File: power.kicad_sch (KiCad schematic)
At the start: 32 parts, among them U2 XC6193A103ER-G, U3 TPS631000DRLR, U4 TPS62840DLCR, U5 BQ25185DLHR

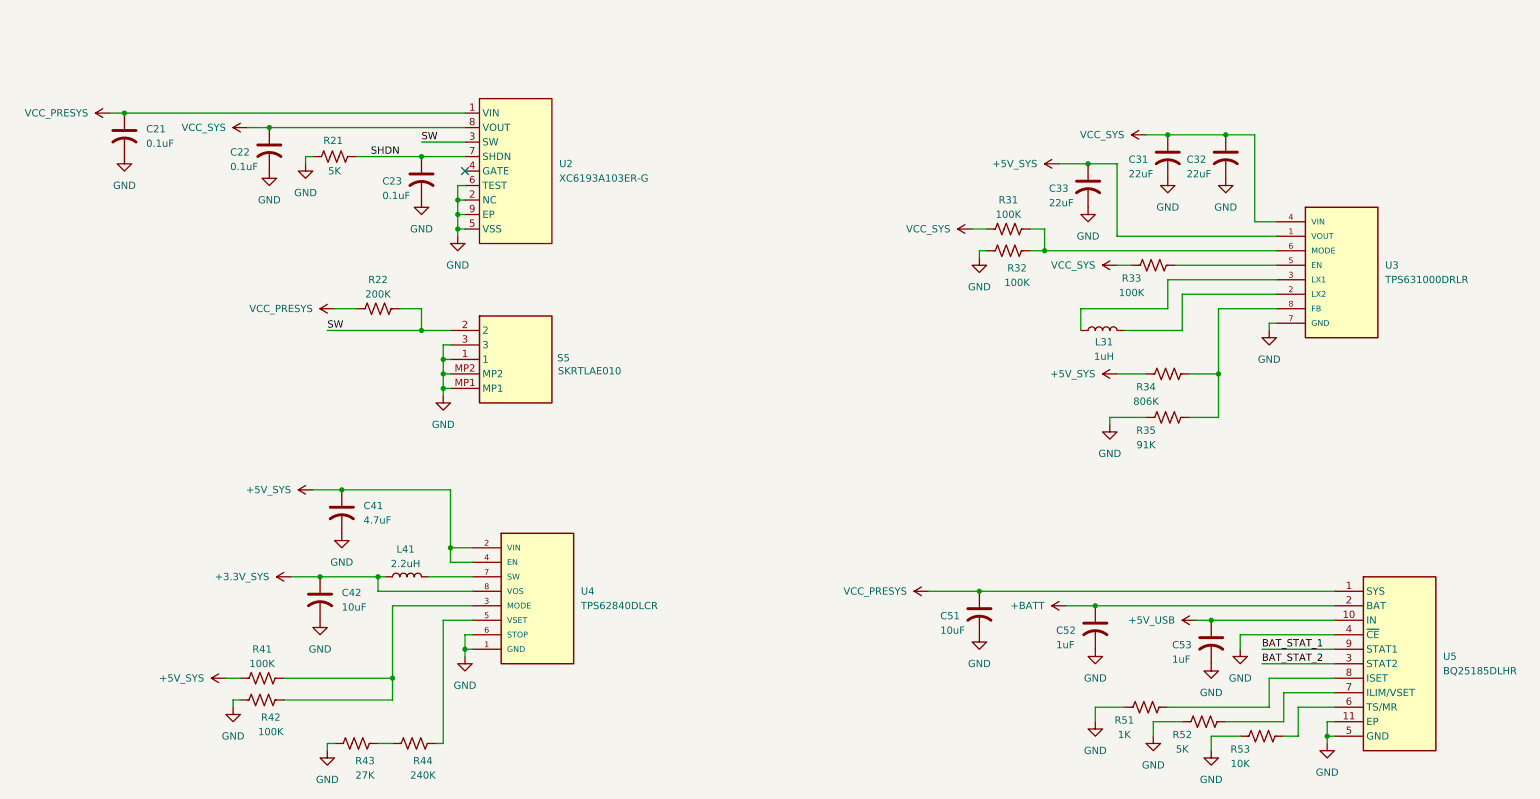
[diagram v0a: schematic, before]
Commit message: Update
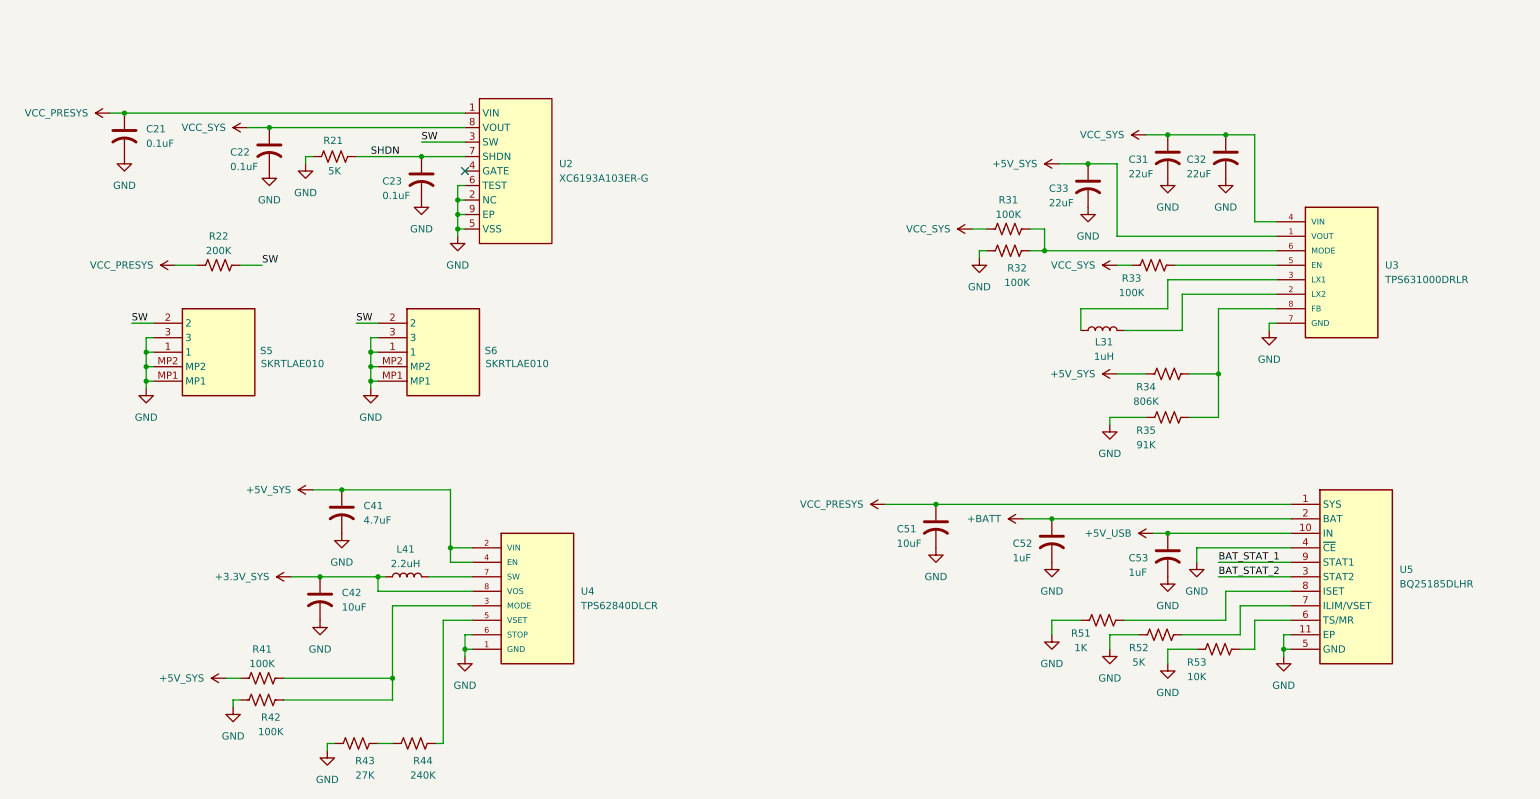
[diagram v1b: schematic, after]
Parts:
- added S6: SKRTLAE010, footprints:SKRTLAE010, symbol SKRTLAE010:SKRTLAE010
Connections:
- net GND: now also S6.1, S6.3, S6.MP1, S6.MP2
- net SW: now also S6.2
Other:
- moved on the sheet: C51, C52, C53, R22, R51, R52, R53, S5, U5

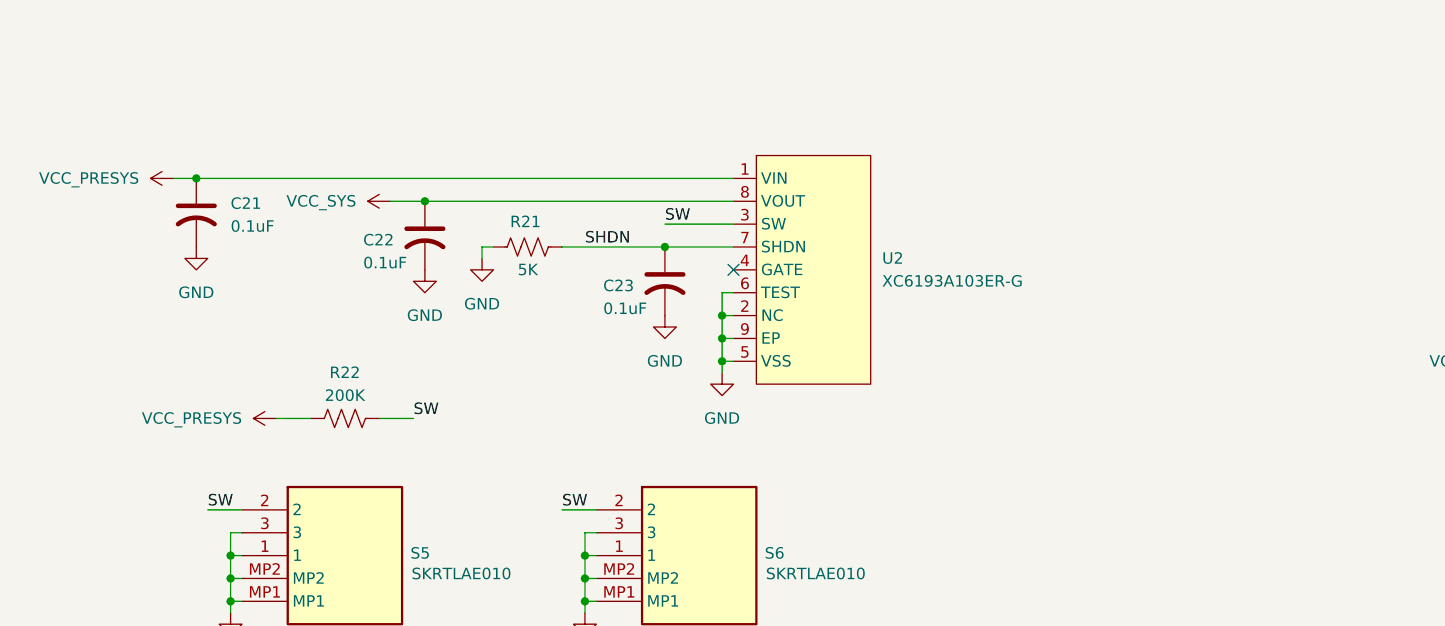
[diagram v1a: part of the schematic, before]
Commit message: Update
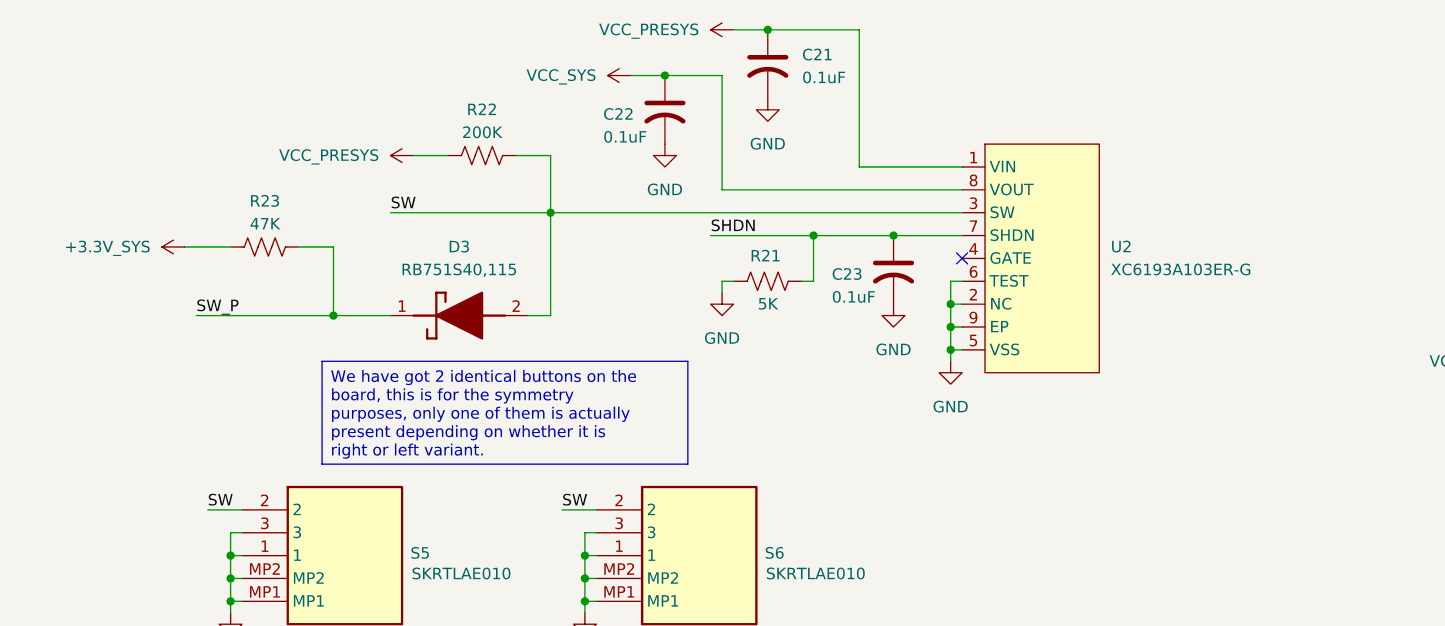
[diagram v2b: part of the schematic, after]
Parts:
- added D3: RB751S40,115, footprints:RB751S40115, symbol RB751S40_115:RB751S40,115
- added R23: 47K, Resistor_SMD:R_0402_1005Metric, symbol Device:R_US
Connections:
- net +3.3V_SYS: now also R23.2
- net SW: now also D3.2 (A)
- new net SW_P: D3.1 (K), R23.1
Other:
- moved on the sheet: C21, C22, C23, R21, R22, U2
